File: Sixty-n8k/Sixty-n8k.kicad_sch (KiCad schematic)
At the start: 67 parts, among them J1 USB4085-GF-A_REVB, J2 SD_CARD_PORT, J3 Conn_02x32_Odd_Even, J4 Conn_01x02, SW1 RESET, SW2 DEBUG, U1 74LS05, U10 74HC164, U11 74LS393, U12 22V10C, U13 74LS148, U14 MC68901P, U16 74LS138, U17 CH340C, U19 74LS21, U2 NE555P, U3 AM29F040-70, U4 AS6C4008, U6 68000D, U7 AS6C4008, U8 AM29F040-70, U9 TPD4E1U06DBVR, X1 7.3728Mhz

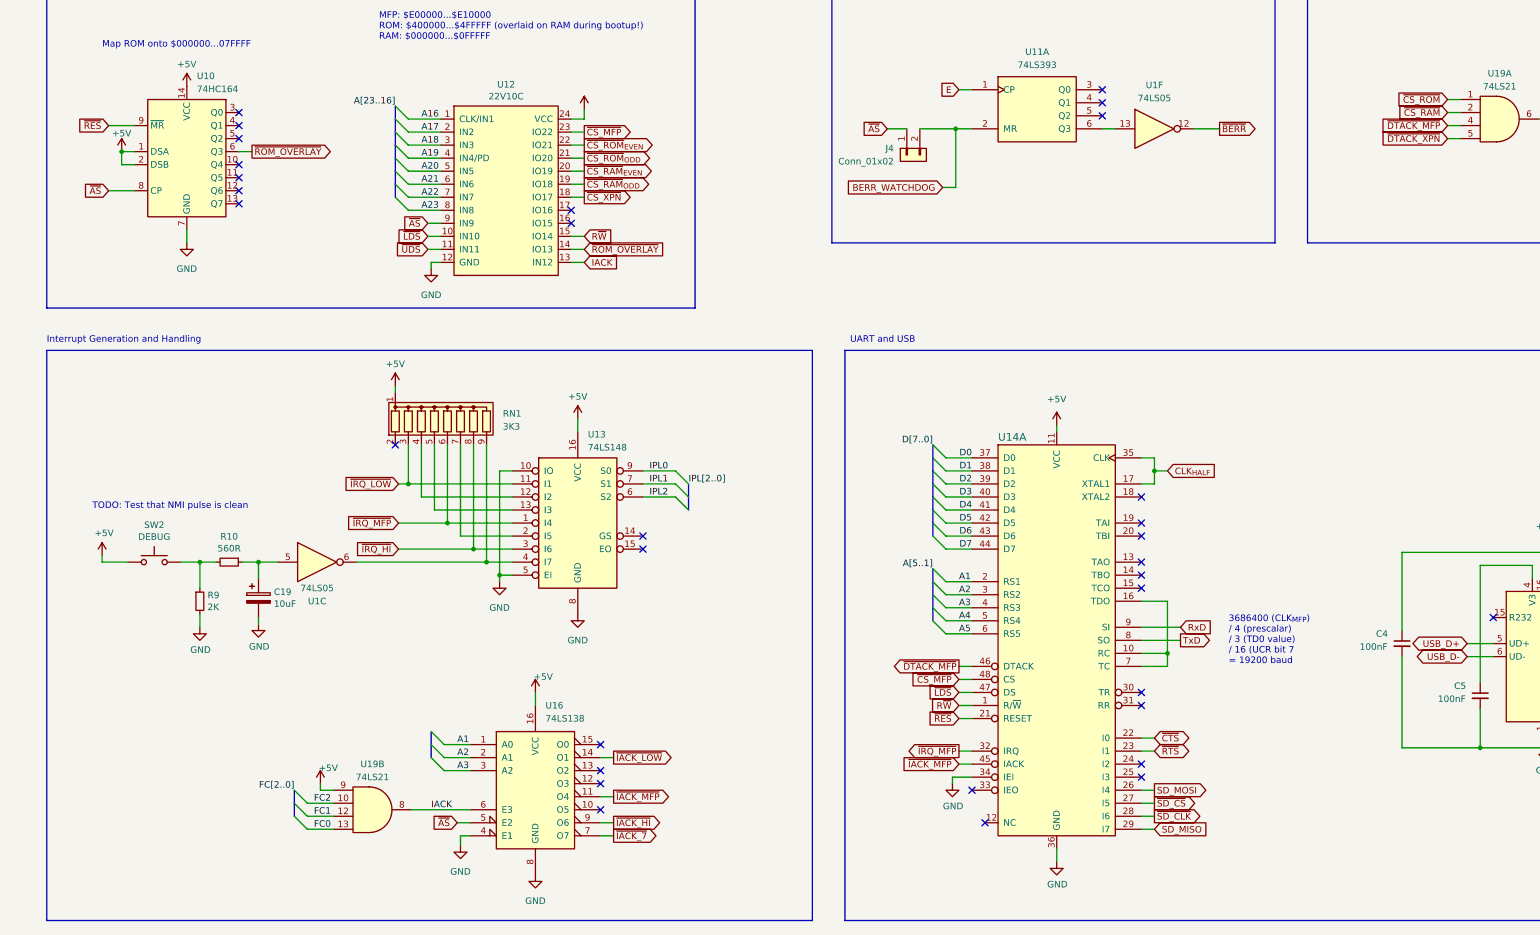
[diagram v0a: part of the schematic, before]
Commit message: RC1
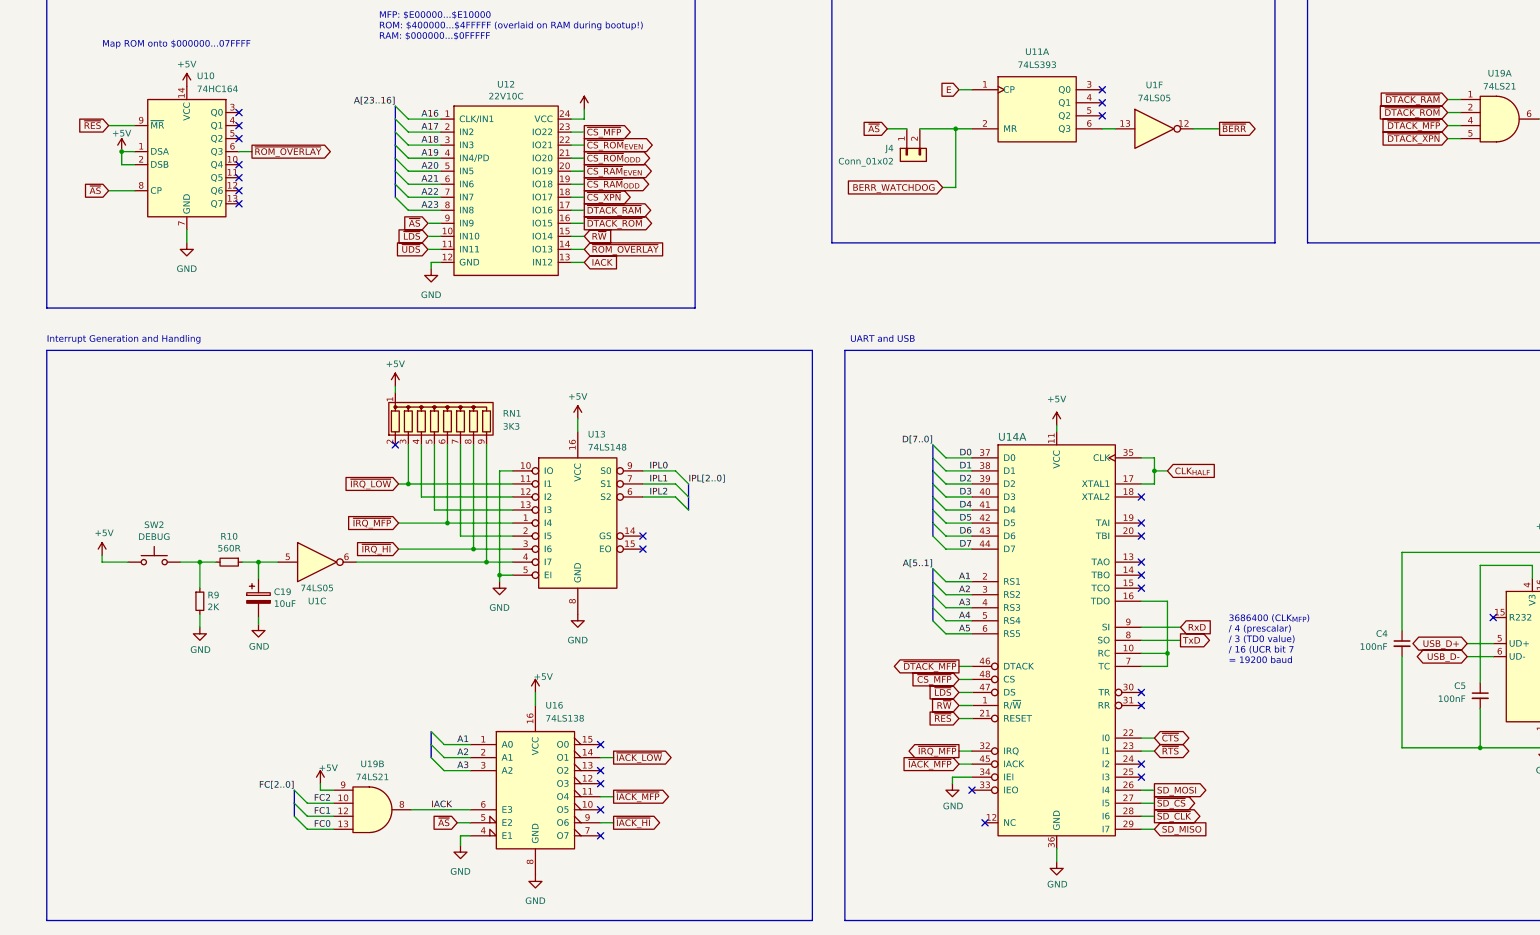
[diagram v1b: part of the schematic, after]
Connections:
- net ~{CS_RAM} is gone; now on net ~{DTACK_ROM}: U19.2
- net ~{CS_ROM} is gone; now on net ~{DTACK_RAM}: U19.1
- net ~{DTACK_ROM}: now reaches U12.16 (IO15)
- net ~{DTACK_RAM}: now reaches U12.17 (IO16)
- net ~{IACK_7}: no longer names the net of U16.7 (O7)
- no-connect marks 54 -> 53
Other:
- note removed: "TODO: Test that NMI pulse is clean"
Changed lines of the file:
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@@
   (no_connect (at 263.525 331.47))
   (no_connect (at 193.04 198.12))
-  (no_connect (at 257.81 217.17))
   (no_connect (at 368.935 283.21))
   (no_connect (at 368.935 270.51))
@@
   (no_connect (at 368.935 285.75))
   (no_connect (at 368.935 275.59))
+  (no_connect (at 263.525 336.55))
   (no_connect (at 539.115 198.755))
   (no_connect (at 368.935 311.15))
@@
   (no_connect (at 271.78 278.13))
   (no_connect (at 361.315 196.215))
-  (no_connect (at 257.81 214.63))
   (no_connect (at 437.515 294.005))
   (no_connect (at 193.04 208.28))
@@
     (stroke (width 0) (type default))
   )
+  (wire (pts (xy 257.81 217.17) (xy 260.35 217.17))
+    (stroke (width 0) (type default))
+  )
   (bus (pts (xy 223.52 194.31) (xy 223.52 196.85))
     (stroke (width 0) (type default))
@@
     (stroke (width 0) (type default))
   )
+  (wire (pts (xy 428.625 195.58) (xy 431.165 195.58))
+    (stroke (width 0) (type default))
+  )
   (wire (pts (xy 243.84 385.445) (xy 243.84 398.145))
     (stroke (width 0) (type default))
@@
     (stroke (width 0) (type default))
   )
+  (wire (pts (xy 257.81 214.63) (xy 260.35 214.63))
+    (stroke (width 0) (type default))
+  )
   (wire (pts (xy 265.43 53.34) (xy 270.51 53.34))
     (stroke (width 0) (type default))
@@
     (stroke (width 0) (type default))
   )
-  (wire (pts (xy 428.625 193.04) (xy 431.165 193.04))
-    (stroke (width 0) (type default))
-  )
   (wire (pts (xy 447.04 43.18) (xy 452.12 43.18))
     (stroke (width 0) (type default))
@@
     (stroke (width 0) (type default))
   )
-  (wire (pts (xy 428.625 195.58) (xy 431.165 195.58))
-    (stroke (width 0) (type default))
-  )
   (wire (pts (xy 265.43 96.52) (xy 270.51 96.52))
     (stroke (width 0) (type default))
@@
     (stroke (width 0) (type default))
   )
-  (wire (pts (xy 263.525 336.55) (xy 266.065 336.55))
-    (stroke (width 0) (type default))
-  )
   (wire (pts (xy 265.43 121.92) (xy 270.51 121.92))
     (stroke (width 0) (type default))
@@
     (stroke (width 0) (type default))
   )
+  (wire (pts (xy 428.625 193.04) (xy 431.165 193.04))
+    (stroke (width 0) (type default))
+  )
   (wire (pts (xy 238.76 260.35) (xy 238.76 280.67))
     (stroke (width 0) (type default))
@@
     (effects (font (size 1.27 1.27)) (justify left bottom))
   )
-  (text "TODO: Test that NMI pulse is clean" (at 164.465 273.05 0)
-    (effects (font (size 1.27 1.27)) (justify left bottom))
-  )
   (text "Address Decoding" (at 155.575 166.37 0)
     (effects (font (size 1.27 1.27)) (justify left bottom))
@@
     )
   )
+  (global_label "~{DTACK_RAM}" (shape output) (at 260.35 214.63 0) (fields_autoplaced)
+    (effects (font (size 1.27 1.27)) (justify left))
+    (property "Intersheetrefs" "${INTERSHEET_REFS}" (at 273.8996 214.63 0)
+      (effects (font (size 1.27 1.27)) (justify left) hide)
+    )
+  )
   (global_label "CLK_{CPU}" (shape input) (at 212.09 35.56 180) (fields_autoplaced)
     (effects (font (size 1.27 1.27)) (justify right))
@@
     )
   )
+  (global_label "~{DTACK_RAM}" (shape input) (at 428.625 193.04 180) (fields_autoplaced)
+    (effects (font (size 1.27 1.27)) (justify right))
+    (property "Intersheetrefs" "${INTERSHEET_REFS}" (at 415.0754 193.04 0)
+      (effects (font (size 1.27 1.27)) (justify right) hide)
+    )
+  )
   (global_label "~{IRQ_MFP}" (shape input) (at 224.155 275.59 180) (fields_autoplaced)
     (effects (font (size 1.27 1.27)) (justify right))
@@
     )
   )
+  (global_label "~{DTACK_ROM}" (shape output) (at 260.35 217.17 0) (fields_autoplaced)
+    (effects (font (size 1.27 1.27)) (justify left))
+    (property "Intersheetrefs" "${INTERSHEET_REFS}" (at 274.1415 217.17 0)
+      (effects (font (size 1.27 1.27)) (justify left) hide)
+    )
+  )
   (global_label "R~{W}" (shape input) (at 333.375 311.15 180) (fields_autoplaced)
     (effects (font (size 1.27 1.27)) (justify right))
@@
     )
   )
-  (global_label "~{CS_ROM}" (shape input) (at 428.625 193.04 180) (fields_autoplaced)
-    (effects (font (size 1.27 1.27)) (justify right))
-    (property "Intersheetrefs" "${INTERSHEET_REFS}" (at 418.2202 193.04 0)
-      (effects (font (size 1.27 1.27)) (justify right) hide)
-    )
-  )
   (global_label "IACK" (shape input) (at 260.35 224.79 0) (fields_autoplaced)
     (effects (font (size 1.27 1.27)) (justify left))
@@
     )
   )
+  (global_label "~{DTACK_ROM}" (shape input) (at 428.625 195.58 180) (fields_autoplaced)
+    (effects (font (size 1.27 1.27)) (justify right))
+    (property "Intersheetrefs" "${INTERSHEET_REFS}" (at 414.8335 195.58 0)
+      (effects (font (size 1.27 1.27)) (justify right) hide)
+    )
+  )
   (global_label "CLK_{CPU}" (shape output) (at 63.5 203.2 0) (fields_autoplaced)
     (effects (font (size 1.27 1.27)) (justify left))
@@
     )
   )
-  (global_label "~{IACK_7}" (shape output) (at 266.065 336.55 0) (fields_autoplaced)
-    (effects (font (size 1.27 1.27)) (justify left))
-    (property "Intersheetrefs" "${INTERSHEET_REFS}" (at 275.3813 336.55 0)
-      (effects (font (size 1.27 1.27)) (justify left) hide)
-    )
-  )
   (global_label "~{RES}" (shape input) (at 167.64 198.12 180) (fields_autoplaced)
     (effects (font (size 1.27 1.27)) (justify right))
@@
       (effects (font (size 1.27 1.27)) (justify right) hide)
     )
-  )
-  (global_label "~{CS_RAM}" (shape input) (at 428.625 195.58 180) (fields_autoplaced)
-    (effects (font (size 1.27 1.27)) (justify right))
-    (property "Intersheetrefs" "${INTERSHEET_REFS}" (at 418.4621 195.58 0)
-      (effects (font (size 1.27 1.27)) (justify right) hide)
-    )
